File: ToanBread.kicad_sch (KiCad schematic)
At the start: 13 parts, among them J1 PJ-059A, J2 AUDIO_IN, J3 VBias_Out, J4 9V_Out, J5 AUDIO_OUT

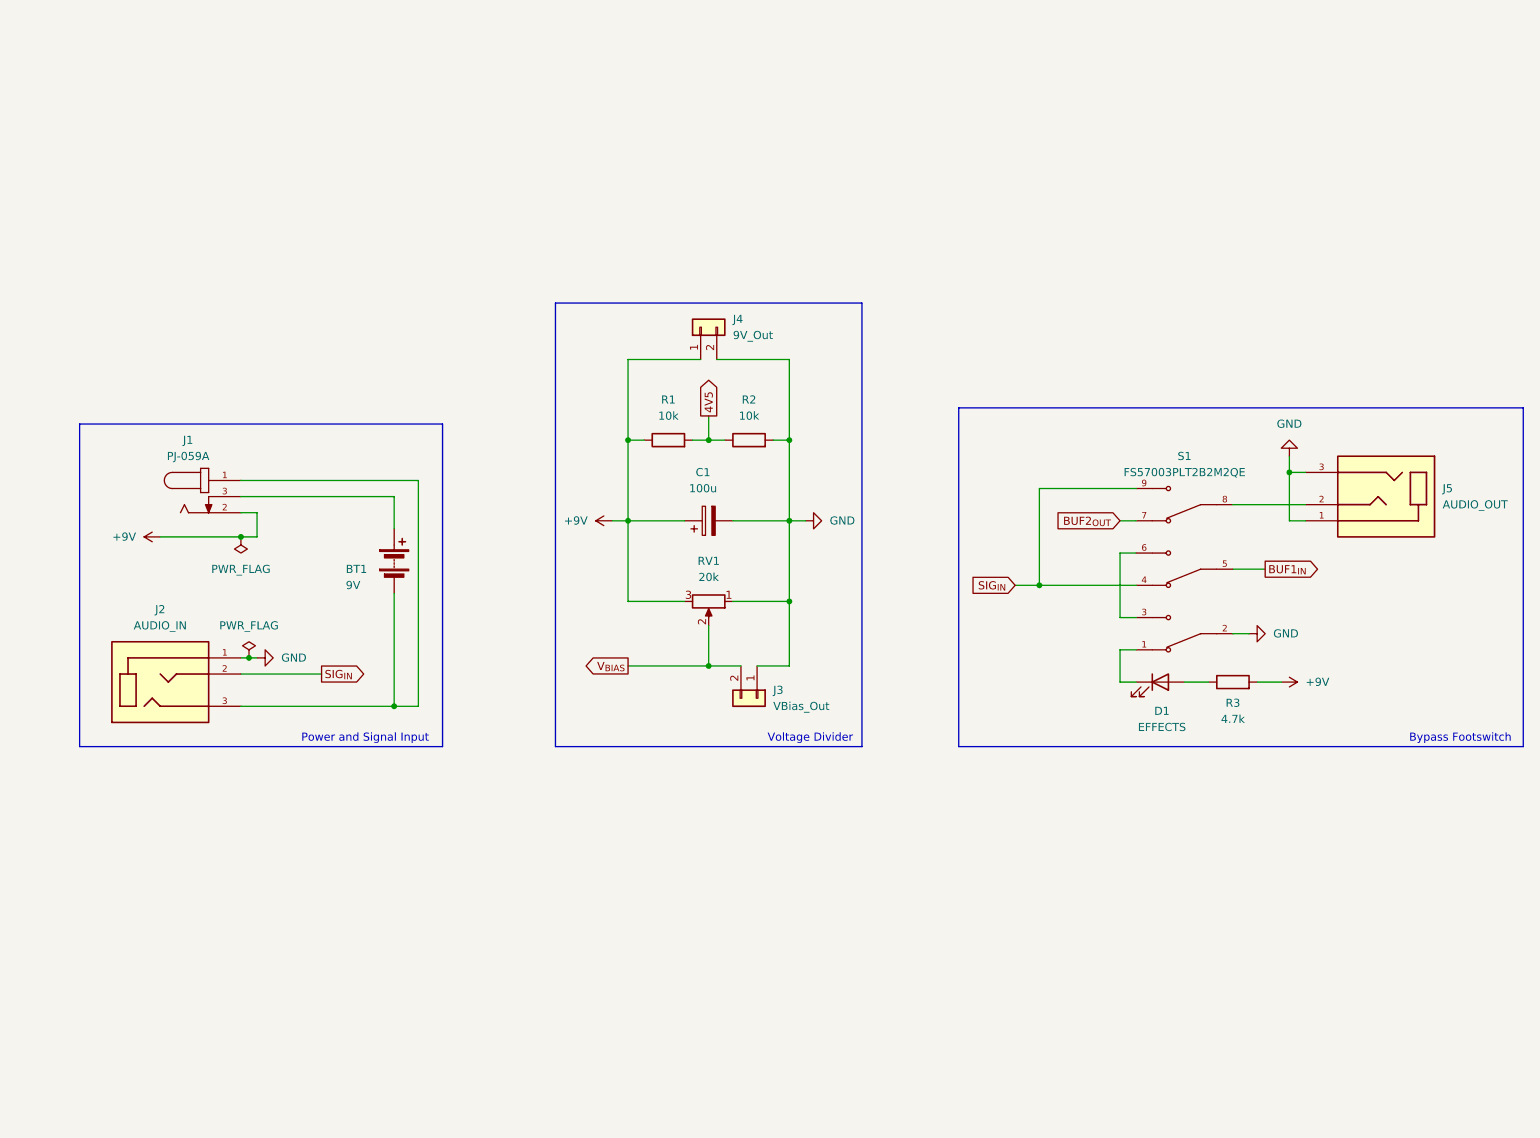
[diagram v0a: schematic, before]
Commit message: Associate most components
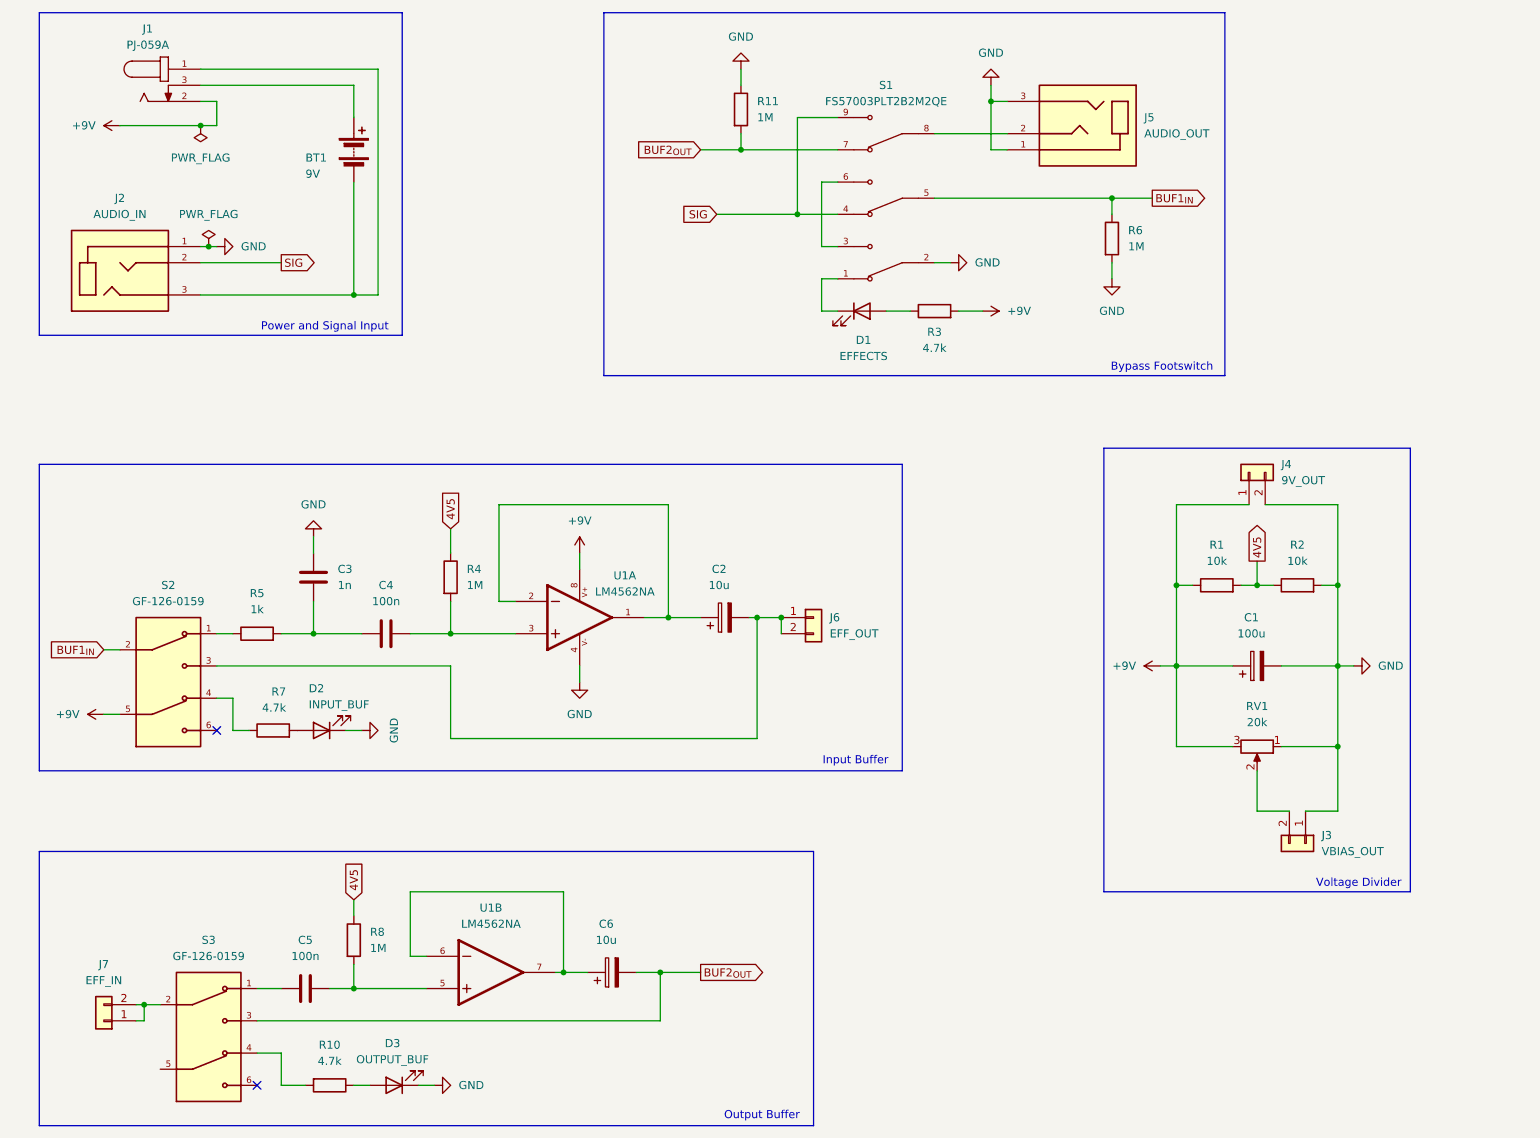
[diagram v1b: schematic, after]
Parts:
- added C2, C6: 10u, Capacitor_THT:CP_Radial_D5.0mm_P2.00mm, symbol Device:C_Polarized
- added C3: 1n, Capacitor_THT:C_Rect_L7.0mm_W2.5mm_P5.00mm, symbol Device:C
- added C4, C5: 100n, Capacitor_THT:C_Rect_L7.0mm_W2.5mm_P5.00mm, symbol Device:C
- added D2: INPUT_BUF, LED_THT:LED_D5.0mm, symbol Device:LED
- added D3: OUTPUT_BUF, LED_THT:LED_D5.0mm, symbol Device:LED
- added J6: EFF_OUT, Connector_PinSocket_2.54mm:PinSocket_1x02_P2.54mm_Vertical, symbol Connector_Generic:Conn_01x02
- added J7: EFF_IN, Connector_PinSocket_2.54mm:PinSocket_1x02_P2.54mm_Vertical, symbol Connector_Generic:Conn_01x02
- added R10, R7: 4.7k, Resistor_THT:R_Axial_DIN0204_L3.6mm_D1.6mm_P5.08mm_Horizontal, symbol Device:R
- added R11, R4, R6, R8: 1M, Resistor_THT:R_Axial_DIN0204_L3.6mm_D1.6mm_P5.08mm_Horizontal, symbol Device:R
- added R5: 1k, Resistor_THT:R_Axial_DIN0204_L3.6mm_D1.6mm_P5.08mm_Horizontal, symbol Device:R
- added S2, S3: GF-126-0159, ProjectSpecific:SW_GF-126-0159, symbol ProjectSpecific:GF-126-0159
- added U1: LM4562NA, ProjectSpecific:DIP794W45P254L959H508Q8, symbol ProjectSpecific:LM4562NA
- BT1, R1: footprint (none) -> Connector_PinSocket_2.54mm:PinSocket_1x02_P2.54mm_Vertical
- C1: footprint (none) -> Capacitor_THT:CP_Radial_D5.0mm_P2.00mm
- D1: footprint (none) -> LED_THT:LED_D5.0mm
- J1: footprint PJ-059A:CUI_PJ-059A -> ProjectSpecific:CUI_PJ-059A
- J2, J5: footprint SJ-63053A:CUI_SJ-63053A -> ProjectSpecific:CUI_SJ-63053A
- J3: value VBias_Out -> VBIAS_OUT; footprint (none) -> Connector_PinSocket_2.54mm:PinSocket_1x02_P2.54mm_Vertical
- J4: value 9V_Out -> 9V_OUT; footprint (none) -> Connector_PinSocket_2.54mm:PinSocket_1x02_P2.54mm_Vertical
- R2, R3: footprint (none) -> Resistor_THT:R_Axial_DIN0204_L3.6mm_D1.6mm_P5.08mm_Horizontal
- S1: footprint FS57003PLT2B2M2QE:SW_FS57003PLT2B2M2QE -> ProjectSpecific:SW_FS57003PLT2B2M2QE
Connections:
- net +9V: now also S2.5, U1.8
- net 4V5: now also R4.1, R8.1
- net BUF1_{IN}: now also R6.1, S2.2
- net BUF2_{OUT}: now also C6.2, R11.2, S3.3
- net GND: now also C3.1, D2.1 (K), D3.1 (K), R11.1, R6.2, U1.4
- net SIG_{IN} renamed SIG
- net V_{BIAS}: no longer names the net of J3.2 (Pin_2), RV1.2
- new net: D3.2 (A), R10.1
- new net: J7.1 (Pin_1), J7.2 (Pin_2), S3.2
- new net: R10.2, S3.4
- new net: R5.1, S2.1
- new net: C2.2, J6.1 (Pin_1), J6.2 (Pin_2), S2.3
- new net: R7.1, S2.4
- new net: C3.2, C4.1, R5.2
- new net: C5.2, R8.2, U1.5
- new net: C6.1, U1.6, U1.7
- new net: C2.1, U1.1, U1.2
- new net: D2.2 (A), R7.2
- new net: C4.2, R4.2, U1.3
- new net: C5.1, S3.1
- no-connect marks 0 -> 2
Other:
- note added: "Input Buffer"
- note added: "Output Buffer"
- moved on the sheet: BT1, C1, D1, J1, J2, J3, J4, J5, R1, R2, R3, RV1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
